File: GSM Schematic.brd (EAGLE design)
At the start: 100.3 x 80 mm, 20 parts, among them J1 5.5x2.1mm Barrel, J2 AVR_SPI_PRG_62X3_LOCK, Q2 16M, U1 ATMEGA328P-PU, U2 LM317MDT-TR

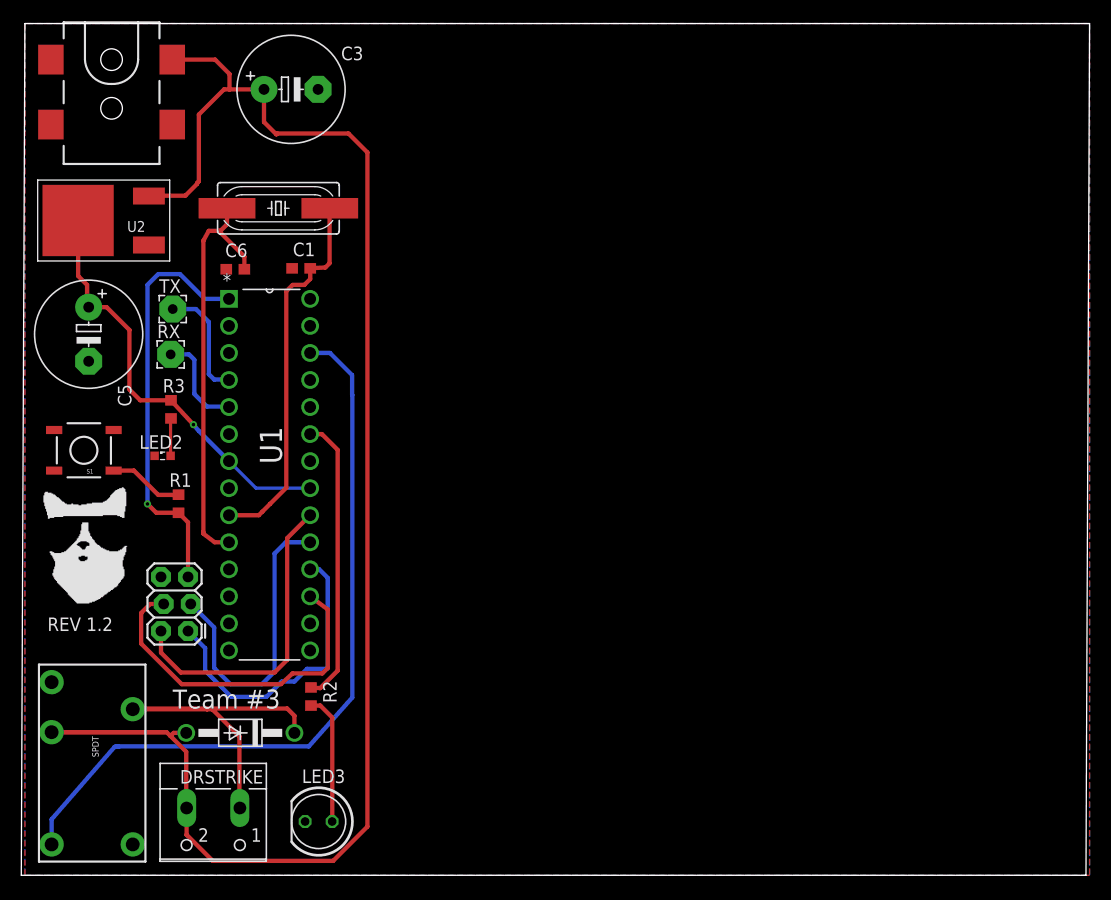
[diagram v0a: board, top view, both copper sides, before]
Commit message: timed and added mounting holes
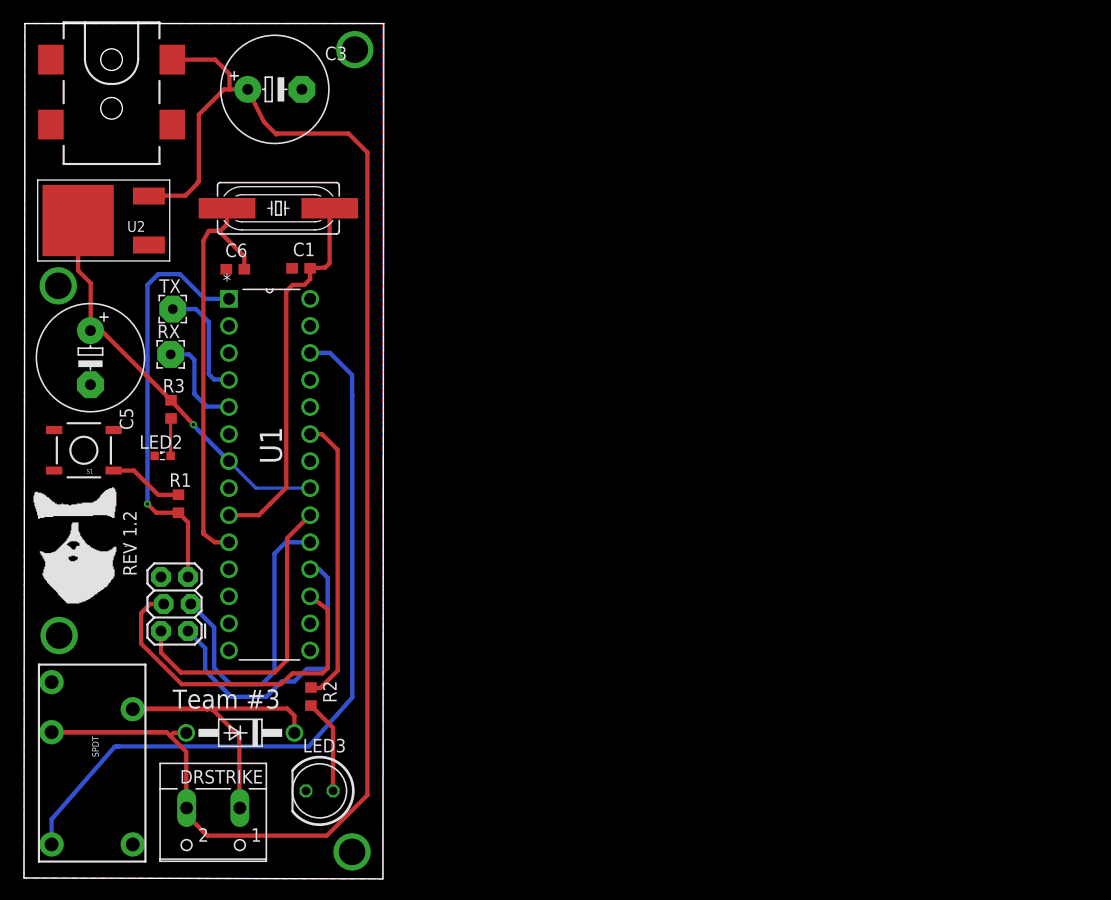
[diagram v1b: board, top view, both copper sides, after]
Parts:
- moved LED3 2.88 mm to (27.7, 7.93)
- moved C5 2.21 mm to (6.16, 48.6)
- moved C3 1.52 mm to (23.5, 73.8)
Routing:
- net 12V: track 156.9 -> 150.9 mm
- net N$6: track 12.2 -> 8.87 mm
- net 5V: track 69.4 -> 67.3 mm
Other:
- board size 100.3 x 80 mm -> 33.8 x 80.3 mm
